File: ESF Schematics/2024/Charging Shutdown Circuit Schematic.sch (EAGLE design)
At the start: 33 parts, among them J1 CONNECTOR-1_6MM2, J10 CONNECTOR-1_CT2242-2, J11 CONNECTOR-5_1-2393947-1, J12 CONNECTOR-3_XXC106-EV-P3Z, J15 CONNECTOR-3_NEMA-5-20, J16 CONNECTOR-3_NEMA-5-20, J17 CONNECTOR-2_, J18 CONNECTOR-2_, J2 CONNECTOR-1_LCAX2-14F-E, J3 CONNECTOR-1_6MM2, J4 CONNECTOR-1_LCAX2-14F-E, J5 CONNECTOR-3_XXC106-EV-P3Z, J6 RING_TERMINAL_19054-0042, J7 RING_TERMINAL_19054-0042, J8 CONNECTOR-3_NEMA-5-20, J9 CONNECTOR-1_CT2242-2

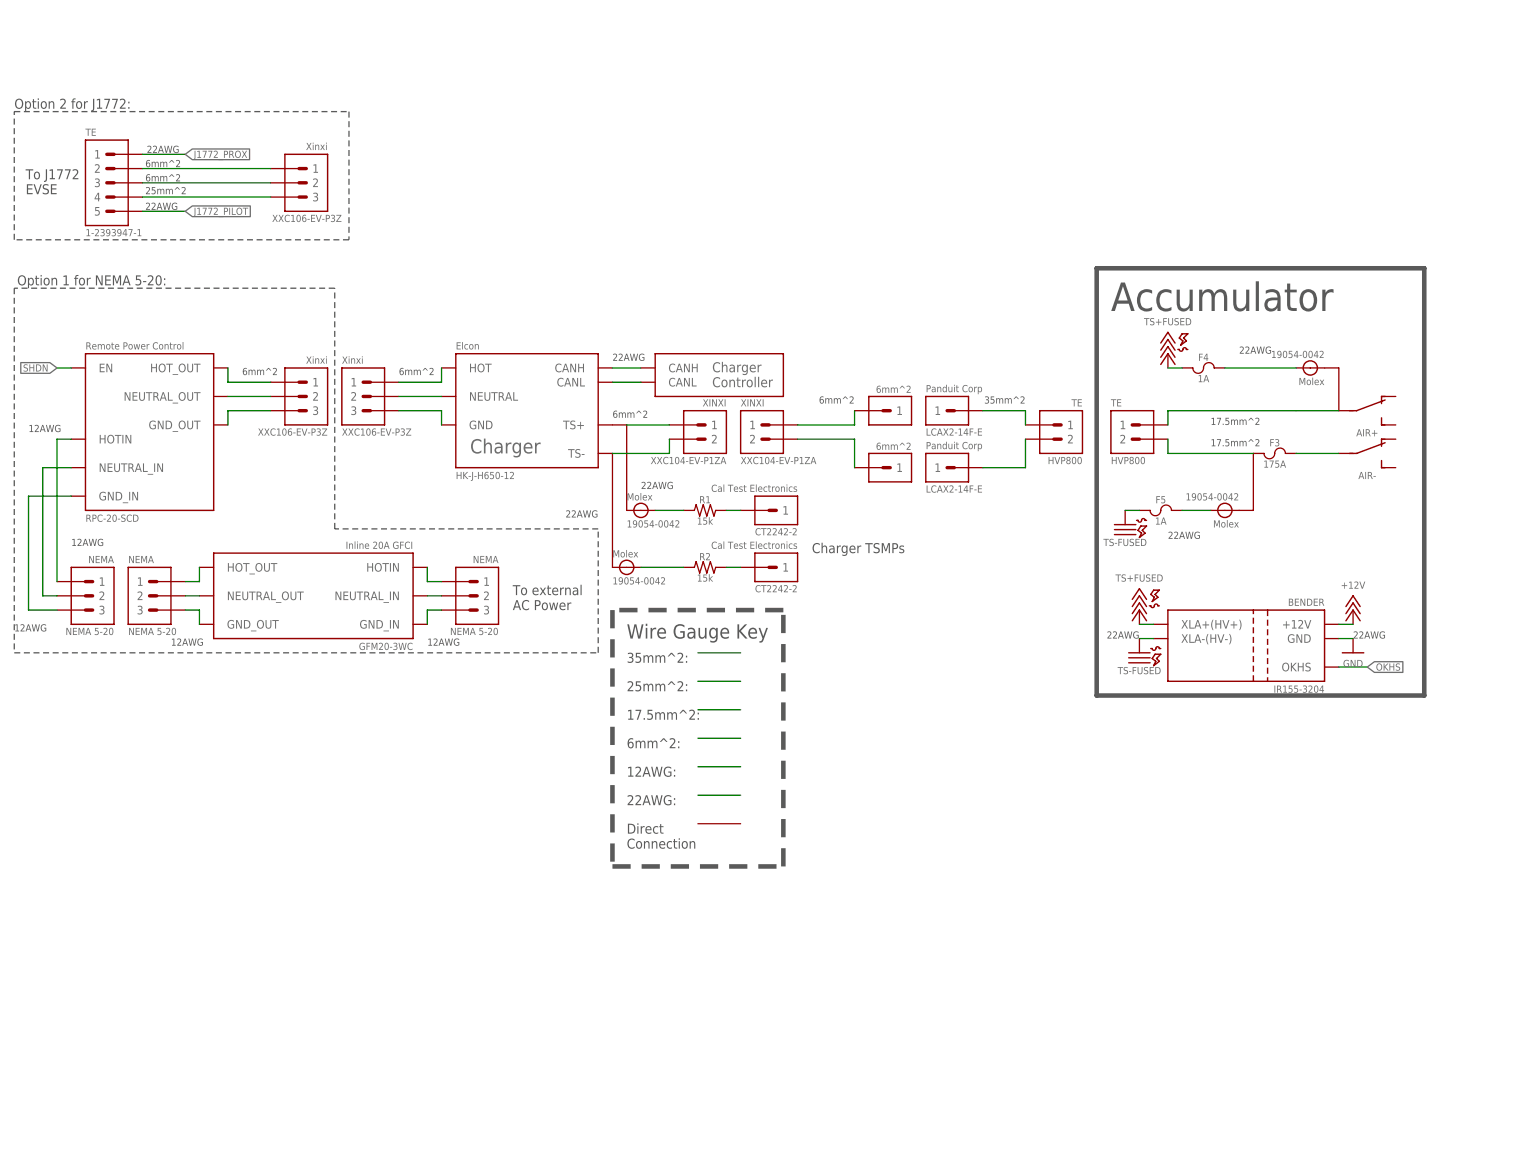
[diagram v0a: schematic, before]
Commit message: num num
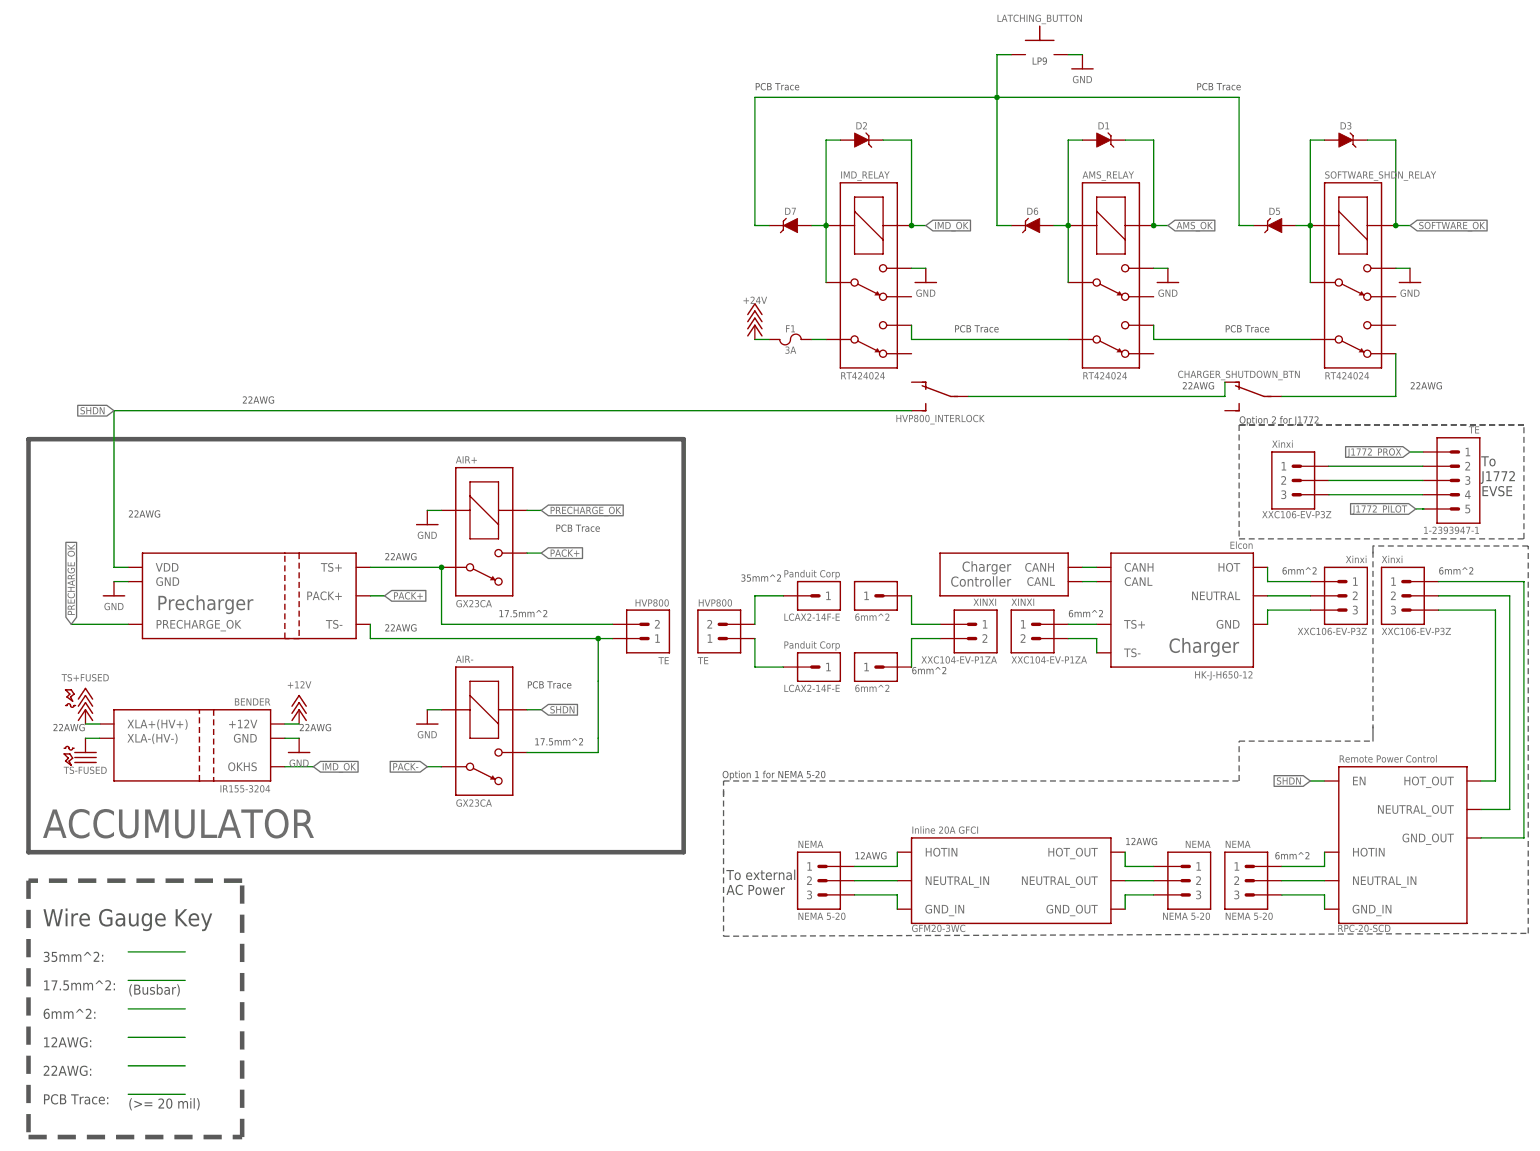
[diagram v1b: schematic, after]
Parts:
- removed F3: 175A, HyTechSymbolsTemp:FUSE
- removed F4, F5: 1A, HyTechSymbolsTemp:FUSE
- removed J12, U$3: CONNECTOR-3_XXC106-EV-P3Z, HyTechSymbols:CONNECTOR-3_XXC106-EV-P3Z
- removed J18: CONNECTOR-2_, HyTechSymbols:CONNECTOR-2_XXC104-EV-P1ZA
- removed R1, R2: 15k, HyTechSymbolsTemp:RESISTOR
- removed S2: SWITCH_SPST_, HyTechSymbols:SWITCH_SPST_
- removed U$1, U$4: CONNECTOR-2_HVP800, HyTechSymbols:CONNECTOR-2_HVP800
- removed U$15: CHARGER_CONTROLLER, HyTechSymbolsTemp:CHARGER_CONTROLLER
- removed U$5: BENDER_IR155-3204, HyTechSymbols:BENDER_IR155-3204
- removed U$6: RING_TERMINAL_19054-0042, HyTechSymbolsTemp:RING_TERMINAL_19054-0042
- added AIR+, AIR-: RELAY_SPST_NO_, HyTechSymbols:RELAY_SPST_NO_
- added AMS_RELAY, IMD_RELAY, SOFTWARE_SHDN_RELAY: RELAY_DPDT_RT424024, HyTechSymbols:RELAY_DPDT_RT424024
- added D1, D2, D3, D5, D6, D7: DIODE, HyTechSymbolsTemp:DIODE
- added F1: 3A, HyTechSymbolsTemp:FUSE
- added J14: CONNECTOR-3_NEMA-5-20, HyTechSymbolsTemp:CONNECTOR-3_NEMA-5-20
- added LATCHING_BUTTON: BUTTON_NO_LP9, HyTechSymbolsTemp:BUTTON_NO_LP9
- added S3: SWITCH_SPST_, HyTechSymbols:SWITCH_SPST_
- added U$11: CHARGER_CONTROLLER, HyTechSymbolsTemp:CHARGER_CONTROLLER
- added U$12: BENDER_IR155-3204, HyTechSymbols:BENDER_IR155-3204
- A1: value REMOTE_POWER_CONTROL_RPC-20-SCD -> INLINE_GFCI_GFM20-3WC; device HyTechSymbolsTemp:REMOTE_POWER_CONTROL_RPC-20-SCD -> HyTechSymbolsTemp:INLINE_GFCI_GFM20-3WC
- A2: value CHARGER_HK-J-H650-12 -> REMOTE_POWER_CONTROL_RPC-20-SCD; device HyTechSymbols:CHARGER_HK-J-H650-12 -> HyTechSymbolsTemp:REMOTE_POWER_CONTROL_RPC-20-SCD
- A3: value INLINE_GFCI_GFM20-3WC -> CHARGER_HK-J-H650-12; device HyTechSymbolsTemp:INLINE_GFCI_GFM20-3WC -> HyTechSymbols:CHARGER_HK-J-H650-12
- J10, J9: value CONNECTOR-1_CT2242-2 -> CONNECTOR-3_XXC106-EV-P3Z; device HyTechSymbolsTemp:CONNECTOR-1_CT2242-2 -> HyTechSymbols:CONNECTOR-3_XXC106-EV-P3Z
- J16: value CONNECTOR-3_NEMA-5-20 -> CONNECTOR-2_; device HyTechSymbolsTemp:CONNECTOR-3_NEMA-5-20 -> HyTechSymbols:CONNECTOR-2_XXC104-EV-P1ZA
- J2: value CONNECTOR-1_LCAX2-14F-E -> CONNECTOR-1_6MM2; device HyTechSymbols:CONNECTOR-1_LCAX2-14F-E -> HyTechSymbols:CONNECTOR-1_6MM2
- J3: value CONNECTOR-1_6MM2 -> CONNECTOR-2_HVP800; device HyTechSymbols:CONNECTOR-1_6MM2 -> HyTechSymbols:CONNECTOR-2_HVP800
- J5: value CONNECTOR-3_XXC106-EV-P3Z -> CONNECTOR-2_HVP800; device HyTechSymbols:CONNECTOR-3_XXC106-EV-P3Z -> HyTechSymbols:CONNECTOR-2_HVP800
- J6: value RING_TERMINAL_19054-0042 -> CONNECTOR-1_LCAX2-14F-E; device HyTechSymbols:RING_TERMINAL_19054-0042 -> HyTechSymbols:CONNECTOR-1_LCAX2-14F-E
- J7: value RING_TERMINAL_19054-0042 -> CONNECTOR-3_NEMA-5-20; device HyTechSymbols:RING_TERMINAL_19054-0042 -> HyTechSymbolsTemp:CONNECTOR-3_NEMA-5-20
- J8: value CONNECTOR-3_NEMA-5-20 -> CONNECTOR-3_XXC106-EV-P3Z; device HyTechSymbolsTemp:CONNECTOR-3_NEMA-5-20 -> HyTechSymbols:CONNECTOR-3_XXC106-EV-P3Z
- S1: MPN AIR+ -> CHARGER_SHUTDOWN_BTN
- U$7: value RING_TERMINAL_19054-0042 -> PRECHARGER; device HyTechSymbolsTemp:RING_TERMINAL_19054-0042 -> HyTechSymbolsTemp:PRECHARGER
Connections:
- removed net N$27: R2.1, U$6.P$2
- removed net N$28: A3.HOT_OUT, J8.1
- removed net N$29: A3.GND_OUT, J8.3
- removed net N$30: A3.GND_IN, J16.3
- removed net N$35 (its old number): F4.2, J6.P$2
- removed net N$36 (its old number): F3.2, S2.P
- removed net N$37 (its old number): J11.3, J12.2
- removed net N$9: J10.1, R2.2
- removed net OKHS: U$5.OKHS
- new net AMS_OK: AMS_RELAY.COIL+, D1.C
- new net IMD_OK: D2.C, IMD_RELAY.COIL+, U$12.OKHS
- new net N$13: AIR-.CONTACT2, J5.1, U$7.TS-
- new net N$16: J1.1, J17.1
- new net N$17: J17.2, J2.1
- new net N$18: J10.3, J11.4
- new net N$22: A3.GND, J8.3
- new net N$24: A2.NEUTRAL_IN, J7.2
- new net N$33: A2.GND_OUT, J9.1
- new net N$34: A1.GND_OUT, J14.3
- new net N$40: A3.TS-, J16.2
- new net N$41: J10.1, J11.2
- new net PACK+: AIR+.CONTACT2, U$7.PACK+
- new net PACK-: AIR-.CONTACT1
- new net PRECHARGE_OK: AIR+.COIL-, U$7.PRECHARGE_OK
- new net SOFTWARE_OK: D3.C, SOFTWARE_SHDN_RELAY.COIL+
- net +12V: now also F1.1, U$12.+12V; no longer U$5.+12V
- net CHARGER_CONTROLLER_CANH: now also A3.CANH, U$11.CANH; no longer A2.CANH, U$15.CANH
- net CHARGER_CONTROLLER_CANL: now also A3.CANL, U$11.CANL; no longer A2.CANL, U$15.CANL
- net GND: now also AIR+.COIL+, AIR-.COIL+, AMS_RELAY.4, IMD_RELAY.4, LATCHING_BUTTON.P$2, SOFTWARE_SHDN_RELAY.4, U$12.GND, U$7.GND; no longer U$5.GND
- net N$1: now also D2.A, D7.A, IMD_RELAY.3, IMD_RELAY.COIL-; no longer A2.NEUTRAL, U$3.2
- net N$10: now also AMS_RELAY.5, SOFTWARE_SHDN_RELAY.6; no longer S1.P, U$1.1
- net N$11: now also AMS_RELAY.6, IMD_RELAY.5; no longer F3.1, U$1.2
- net N$12: now also AIR+.CONTACT1, J5.2, U$7.TS+; no longer J11.2, J12.1
- net N$14: now also J3.1, J6.1; no longer J1.1, J18.1
- net N$15: now also A2.HOT_OUT, J9.3; no longer J18.2, J3.1
- net N$19: now also J10.2, J11.3; no longer A1.GND_OUT, J5.3
- net N$2: now also D5.C, D6.C, D7.C, LATCHING_BUTTON.P$1; no longer A2.GND, U$3.3
- net N$20: now also A3.HOT, J8.1; no longer J4.1, U$4.2
- net N$21: now also A3.NEUTRAL, J8.2; no longer J2.1, U$4.1
- net N$23: now also A2.HOTIN, J7.1; no longer A3.NEUTRAL_OUT, J8.2
- net N$25: now also A2.GND_IN, J7.3; no longer R1.1, U$7.P$2
- net N$26: now also A1.HOT_OUT, J14.1; no longer F5.2, J7.P$2
- net N$3: now also AMS_RELAY.3, AMS_RELAY.COIL-, D1.A, D6.A; no longer A2.HOT, U$3.1
- net N$31: now also A1.NEUTRAL_OUT, J14.2; no longer A3.NEUTRAL_IN, J16.2
- net N$32: now also A2.NEUTRAL_OUT, J9.2; no longer A3.HOTIN, J16.1
- net N$39: now also A3.TS+, J16.1; no longer J11.4, J12.3
- net N$4: now also S1.O, S3.P; no longer J17.1
- net N$5: now also D3.A, D5.A, SOFTWARE_SHDN_RELAY.3, SOFTWARE_SHDN_RELAY.COIL-; no longer A2.TS-, J17.2
- net N$6: now also F1.2, IMD_RELAY.6; no longer A1.HOT_OUT, J5.1
- net N$7: now also S1.P, SOFTWARE_SHDN_RELAY.7; no longer A1.NEUTRAL_OUT, J5.2
- net N$8: now also J3.2, J4.1; no longer J9.1, R1.2
- net SHDN: now also A2.EN, AIR-.COIL-, S3.S, U$7.VDD; no longer A1.EN
- net TS+: now also U$12.XLA+(HV+); no longer F4.1, U$5.XLA+(HV+)
- net TS-UNFUSED: now also U$12.XLA-(HV-); no longer F5.1, U$5.XLA-(HV-)
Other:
- note added: "(>= 20 mil)"
- note added: "(Busbar)"
- note added: "ACCUMULATOR"
- note added: "Option 1 for NEMA 5-20"
- note added: "Option 2 for J1772"
- note added: "PCB Trace"
- note added: "PCB Trace:"
- note removed: "25mm^2"
- note removed: "25mm^2:"
- note removed: "Accumulator"
- note removed: "Charger TSMPs"
- note removed: "Direct Connection"
- note removed: "Option 1 for NEMA 5-20:"
- note removed: "Option 2 for J1772:"
